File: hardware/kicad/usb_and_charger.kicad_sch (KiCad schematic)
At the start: 15 parts, among them J2 USB_C_Receptacle_USB2.0, U1 MCP73831-2-OT, U2 USBLC6-2SC6

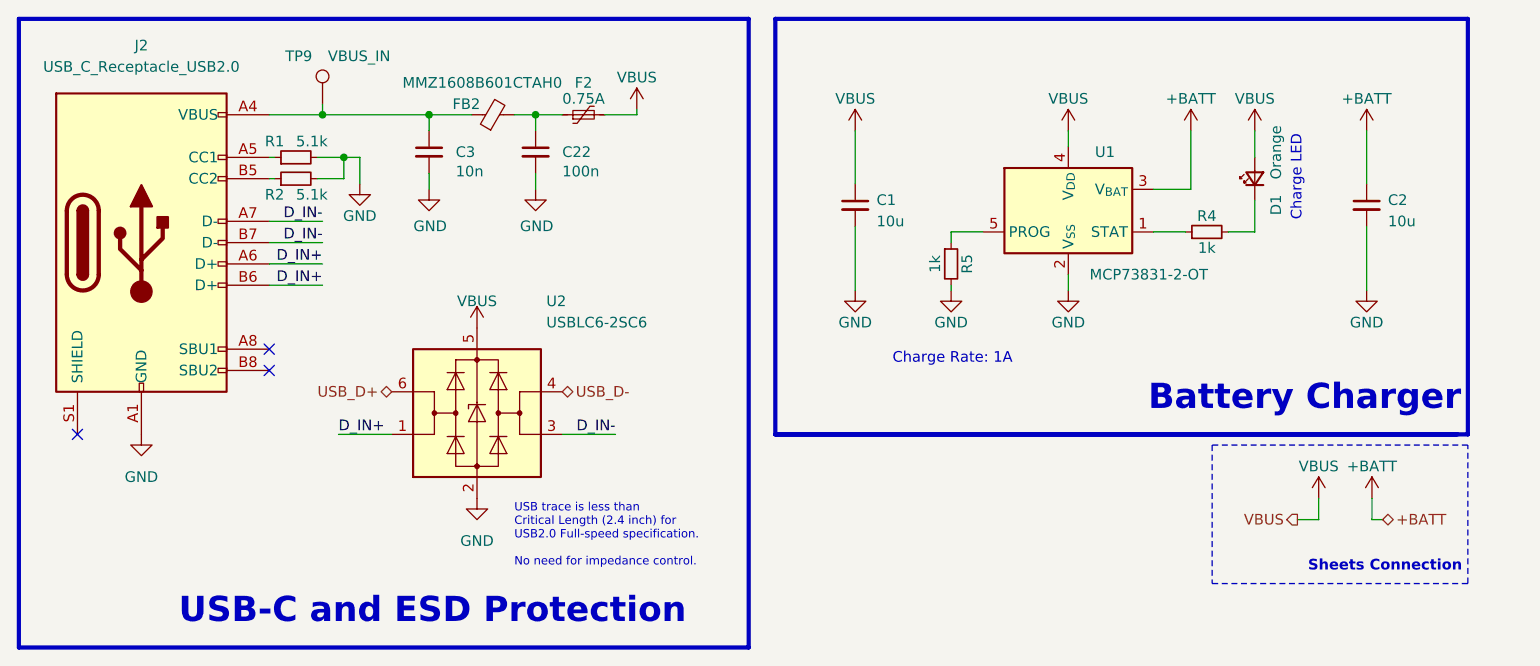
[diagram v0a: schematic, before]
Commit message: wip: revision 2
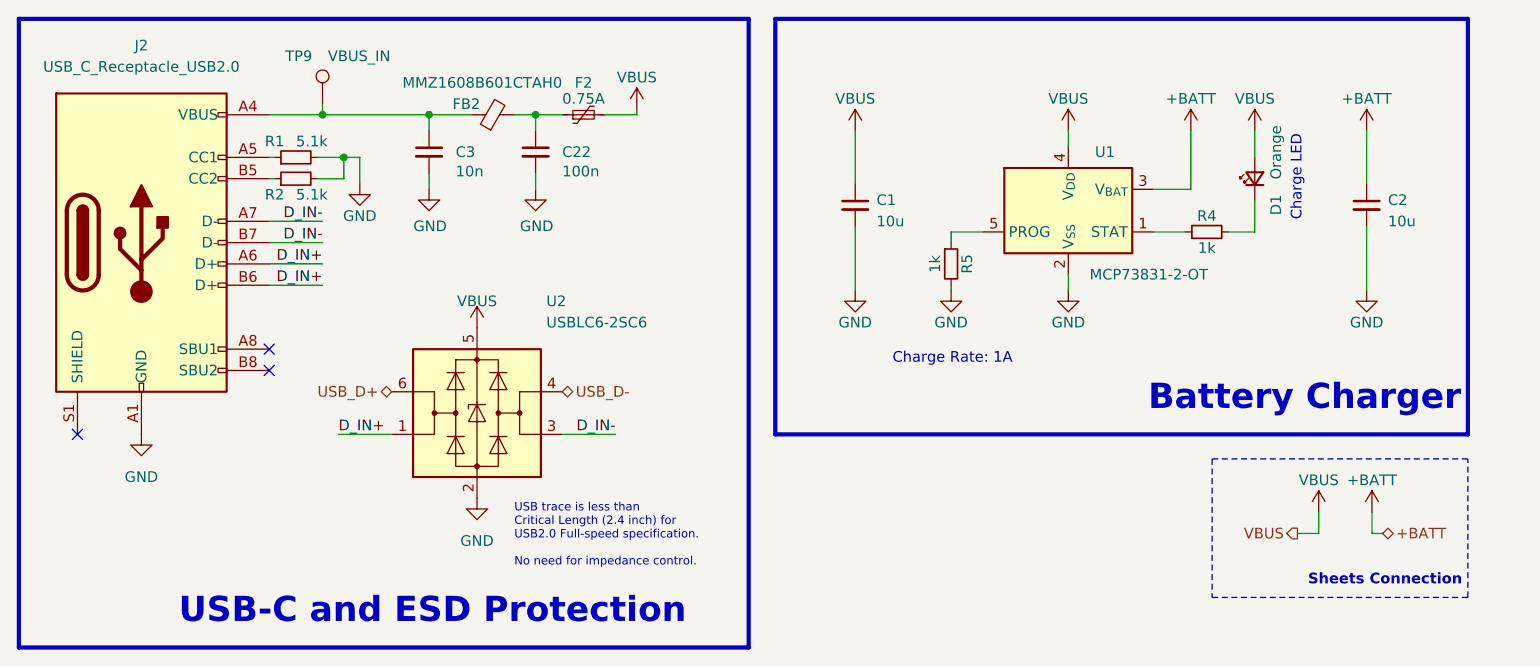
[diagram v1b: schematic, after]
